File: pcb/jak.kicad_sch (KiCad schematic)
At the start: 90 parts, among them SW1 SW_Push, SW10 SW_Push, SW10_r1 SW_Push, SW11 SW_Push, SW11_r1 SW_Push, SW12 SW_Push, SW12_r1 SW_Push, SW13 SW_Push, SW13_r1 SW_Push, SW14 SW_Push, SW14_r1 SW_Push, SW15 SW_Push, SW15_r1 SW_Push, SW16 SW_Push, SW16_r1 SW_Push, SW17 SW_Push, SW17_r1 SW_Push, SW18 SW_Push, SW18_r1 SW_Push, SW1_r1 SW_Push, SW2 SW_Push, SW2_r1 SW_Push, SW3 SW_Push, SW3_r1 SW_Push, SW4 SW_Push, SW4_r1 SW_Push, SW5 SW_Push, SW5_r1 SW_Push, SW6 SW_Push, SW6_r1 SW_Push, SW7 SW_Push, SW7_r1 SW_Push, SW8 SW_Push, SW8_r1 SW_Push, SW9 SW_Push, SW9_r1 SW_Push

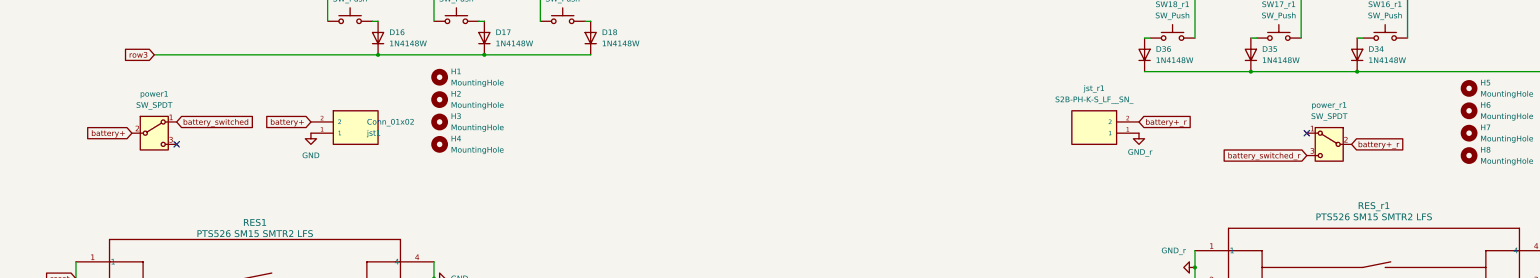
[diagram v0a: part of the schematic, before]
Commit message: Revert "Fixed the power switch pins being swapped and updated the gerber files"
This reverts commit 317bf88c69a0fc961124c453349158f4046b94f1.
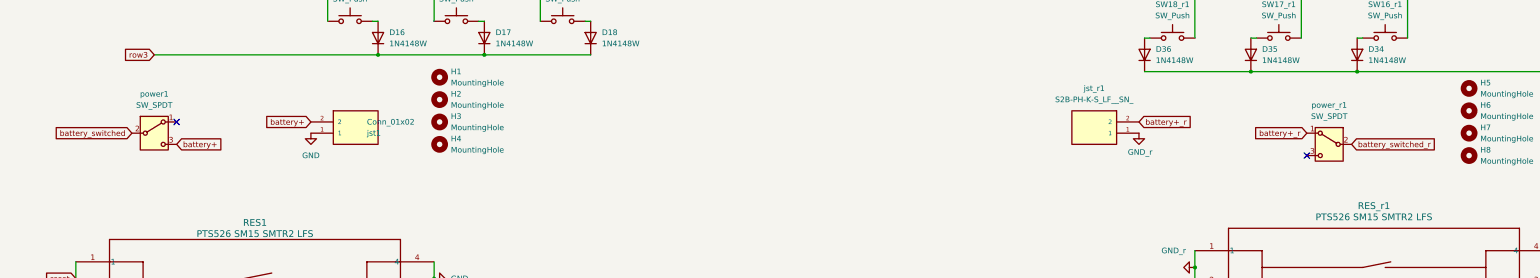
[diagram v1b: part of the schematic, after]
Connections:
- net battery+: now also power1.3 (C); no longer power1.2 (B)
- net battery+_r: now also power_r1.1 (A); no longer power_r1.2 (B)
- net battery_switched: now also power1.2 (B); no longer power1.1 (A)
- net battery_switched_r: now also power_r1.2 (B); no longer power_r1.3 (C)

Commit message: Fixed the power switch pins being swapped and updated the gerber files
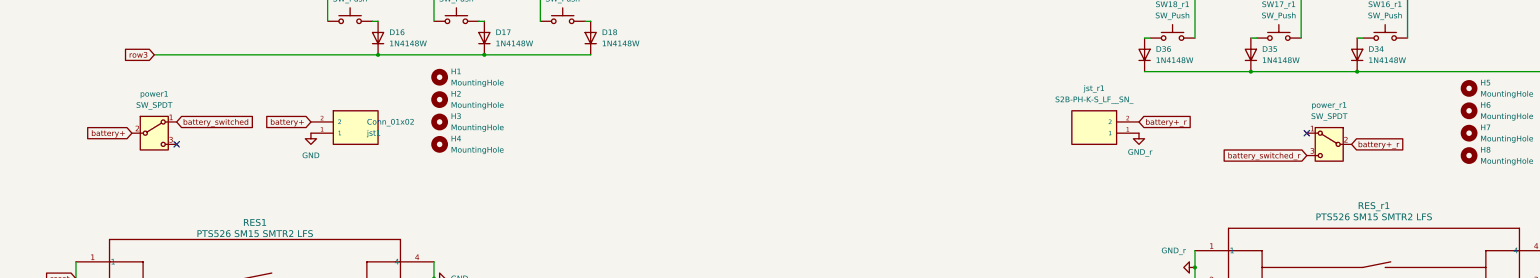
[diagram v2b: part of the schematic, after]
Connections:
- net battery+: now also power1.2 (B); no longer power1.3 (C)
- net battery+_r: now also power_r1.2 (B); no longer power_r1.1 (A)
- net battery_switched: now also power1.1 (A); no longer power1.2 (B)
- net battery_switched_r: now also power_r1.3 (C); no longer power_r1.2 (B)
